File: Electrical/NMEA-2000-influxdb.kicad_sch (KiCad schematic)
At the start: 10 parts, among them J1 Conn_01x02, J2 Conn_01x02, U1 SD-Card-Module, U2 LM7805_TO220, U3 ESP32-DevKitC, U4 SN65HVD230, U5 RTC-Module

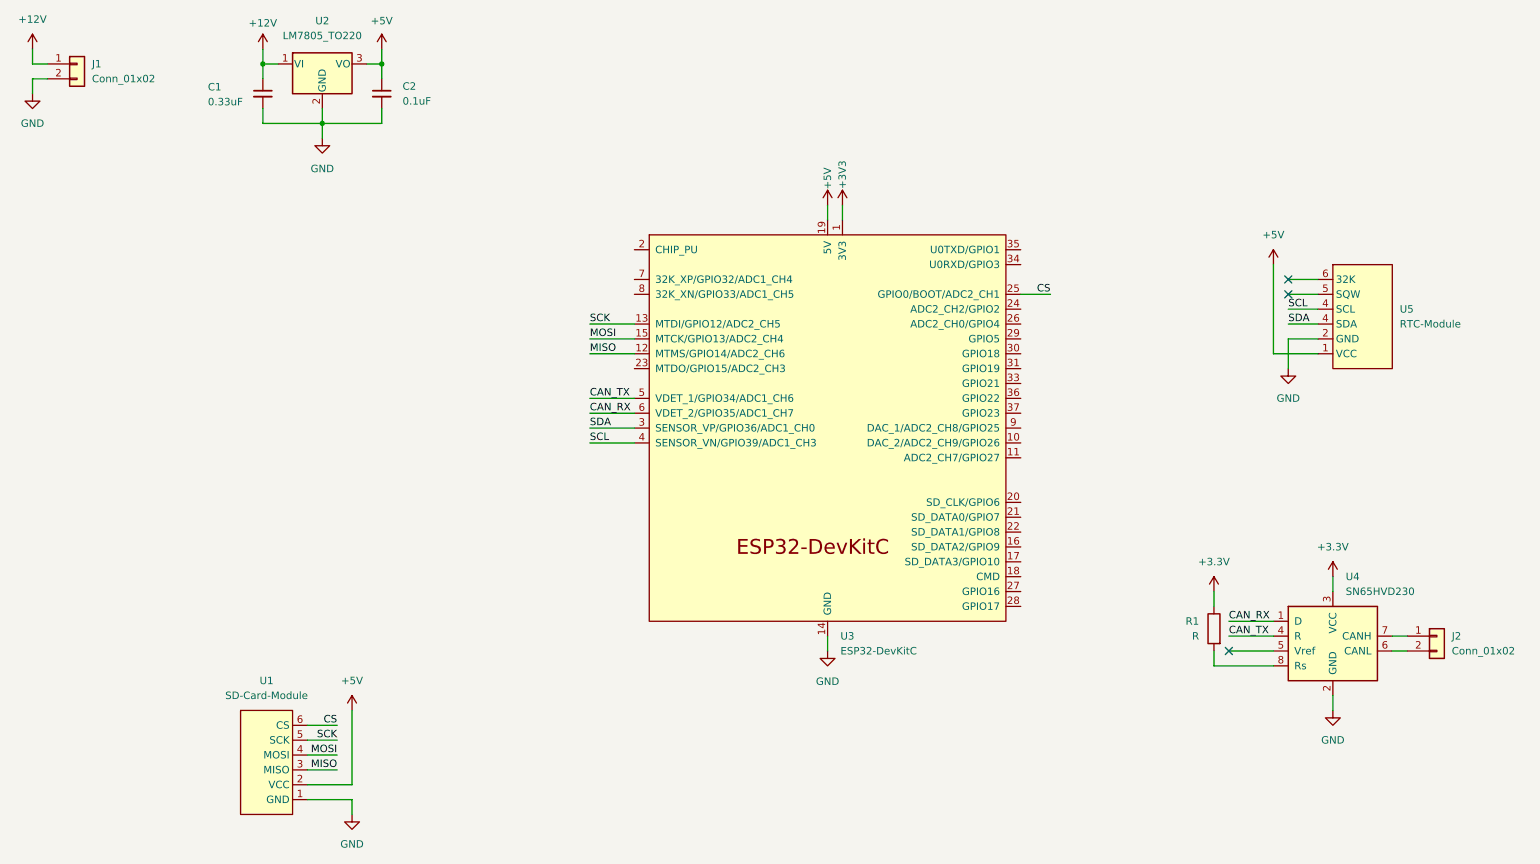
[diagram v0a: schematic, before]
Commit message: Added external connectors
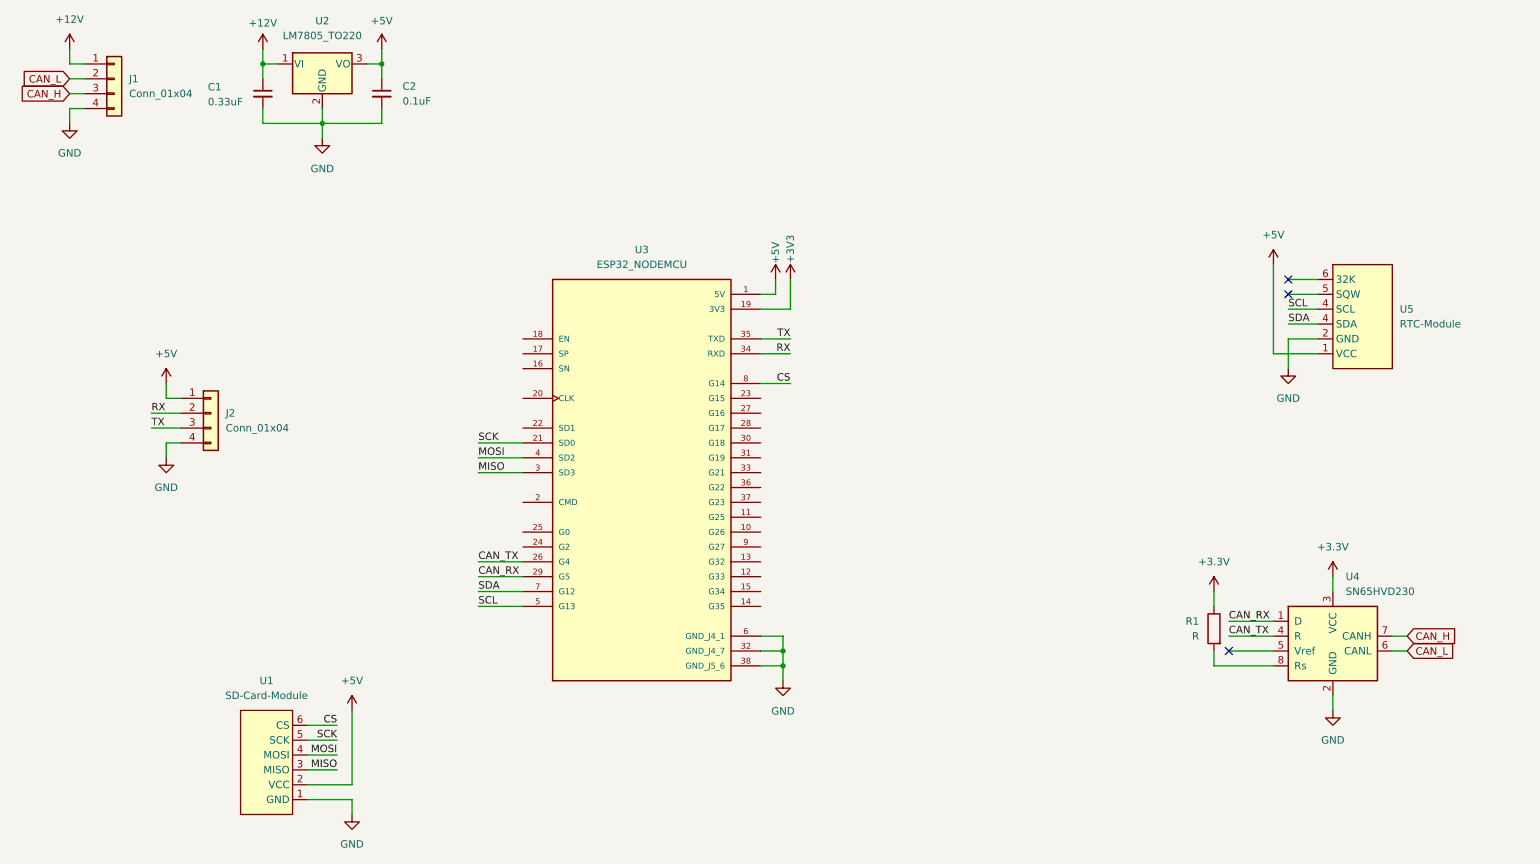
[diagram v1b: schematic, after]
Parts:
- removed J1: Conn_01x02, Capacitor_THT:CP_Radial_D8.0mm_P5.00mm, symbol Connector_Generic:Conn_01x02
- removed J2: Conn_01x02, TerminalBlock_Phoenix:TerminalBlock_Phoenix_MKDS-1,5-2-5.08_1x02_P5.08mm_Horizontal, symbol Connector_Generic:Conn_01x02
- removed U3: ESP32-DevKitC, Espressif:MODULE_ESP32_NODEMCU, symbol Espressif:ESP32-DevKitC
- added J1: Conn_01x04, TerminalBlock_Phoenix:TerminalBlock_Phoenix_MKDS-1,5-4-5.08_1x04_P5.08mm_Horizontal, symbol Connector_Generic:Conn_01x04
- added J2: Conn_01x04, Connector_PinSocket_2.54mm:PinSocket_1x04_P2.54mm_Horizontal, symbol Connector_Generic:Conn_01x04
- added U3: ESP32_NODEMCU, esp32:esp32, symbol ESP32_NODEMCU:ESP32_NODEMCU
- U1, U5: footprint Connector_PinSocket_2.54mm:PinSocket_1x06_P2.54mm_Vertical -> Connector_PinSocket_2.54mm:PinSocket_1x06_P2.54mm_Horizontal
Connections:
- net +12V: now also J1.1 (Pin_1)
- net +3V3: now also U3.19 (3V3)
- net +5V: now also J2.1 (Pin_1), U3.1 (5V)
- net CAN_RX: now also U3.29 (G5)
- net CAN_TX: now also U3.26 (G4)
- net CS: now also U3.8 (G14)
- net GND: now also J1.4 (Pin_4), J2.4 (Pin_4), U3.32 (GND_J4_7), U3.38 (GND_J5_6), U3.6 (GND_J4_1)
- net MISO: now also U3.3 (SD3)
- net MOSI: now also U3.4 (SD2)
- net SCK: now also U3.21 (SD0)
- net SCL: now also U3.5 (G13)
- net SDA: now also U3.7 (G12)
- net CAN_L: now reaches U4.6 (CANL)
- net CAN_L: now also J1.2 (Pin_2)
- net CAN_H: now reaches U4.7 (CANH)
- net CAN_H: now also J1.3 (Pin_3)
- new net RX: J2.2 (Pin_2), U3.34 (RXD)
- new net TX: J2.3 (Pin_3), U3.35 (TXD)
